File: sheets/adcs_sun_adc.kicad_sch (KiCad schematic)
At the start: 1 part, among them U10 MCP3208

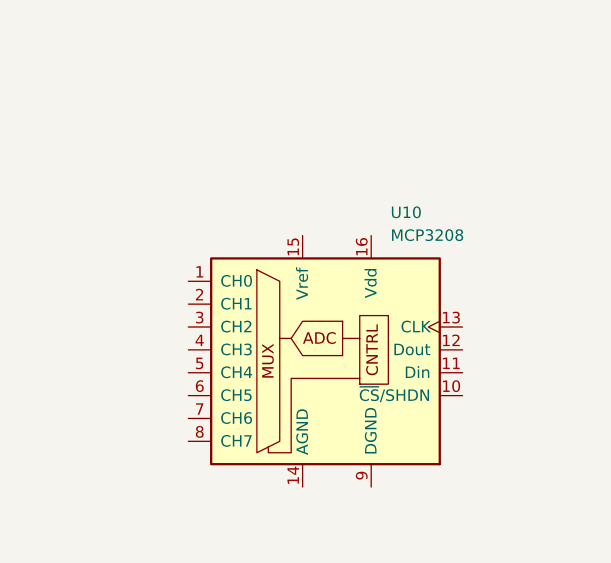
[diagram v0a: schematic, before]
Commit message: push
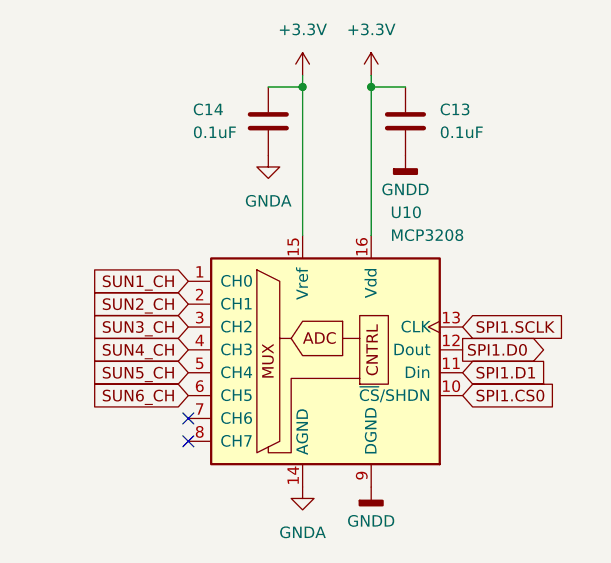
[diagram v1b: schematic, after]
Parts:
- added C13, C14: 0.1uF, symbol Device:C
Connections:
- net SUN1_CH: now reaches U10.1 (CH0)
- net SPI1.CS0: now reaches U10.10 (~{CS}/SHDN)
- net SPI1.D1: now reaches U10.11 (Din)
- net SPI1.D0: now reaches U10.12 (Dout)
- net SPI1.SCLK: now reaches U10.13 (CLK)
- net GNDA: now reaches U10.14 (AGND)
- net GNDA: now also C14.2
- net +3.3V: now reaches U10.15 (Vref)
- net +3.3V: now also U10.16 (Vdd), C13.1, C14.1
- net SUN2_CH: now reaches U10.2 (CH1)
- net SUN3_CH: now reaches U10.3 (CH2)
- net SUN4_CH: now reaches U10.4 (CH3)
- net SUN5_CH: now reaches U10.5 (CH4)
- net SUN6_CH: now reaches U10.6 (CH5)
- net GNDD: now reaches U10.9 (DGND)
- net GNDD: now also C13.2
- no-connect marks 0 -> 2

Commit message: allocating pins ?
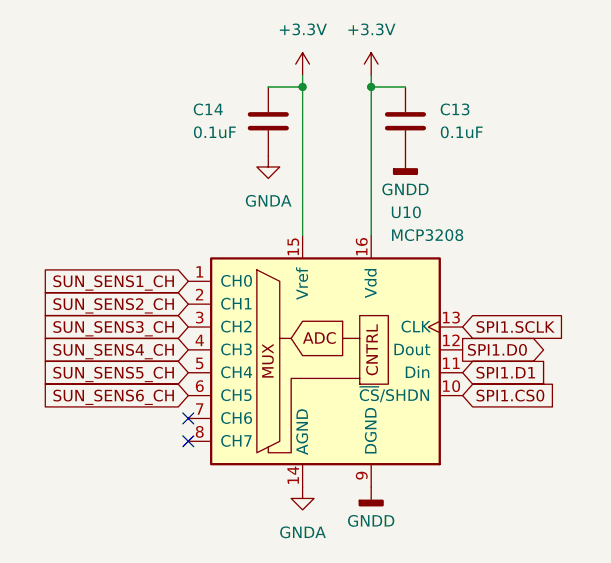
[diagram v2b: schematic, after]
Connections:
- net SUN1_CH renamed SUN_SENS1_CH
- net SUN2_CH renamed SUN_SENS2_CH
- net SUN3_CH renamed SUN_SENS3_CH
- net SUN4_CH renamed SUN_SENS4_CH
- net SUN5_CH renamed SUN_SENS5_CH
- net SUN6_CH renamed SUN_SENS6_CH
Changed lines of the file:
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@@
 		)
 	)
-	(global_label "SUN4_CH"
+	(global_label "SUN_SENS4_CH"
 		(shape input)
 		(at 133.35 91.44 180)
@@
 		)
 		(property "Intersheetrefs" "${INTERSHEET_REFS}"
-			(at 121.6216 91.44 0)
-			(hide yes)
-			(show_name no)
-			(do_not_autoplace no)
-			(effects
-				(font
-					(size 1.27 1.27)
-				)
-				(justify right)
-			)
-		)
-	)
-	(global_label "SUN6_CH"
+			(at 115.7555 91.44 0)
+			(hide yes)
+			(show_name no)
+			(do_not_autoplace no)
+			(effects
+				(font
+					(size 1.27 1.27)
+				)
+				(justify right)
+			)
+		)
+	)
+	(global_label "SUN_SENS6_CH"
 		(shape input)
 		(at 133.35 96.52 180)
@@
 		)
 		(property "Intersheetrefs" "${INTERSHEET_REFS}"
-			(at 121.6216 96.52 0)
-			(hide yes)
-			(show_name no)
-			(do_not_autoplace no)
-			(effects
-				(font
-					(size 1.27 1.27)
-				)
-				(justify right)
-			)
-		)
-	)
-	(global_label "SUN2_CH"
+			(at 115.7555 96.52 0)
+			(hide yes)
+			(show_name no)
+			(do_not_autoplace no)
+			(effects
+				(font
+					(size 1.27 1.27)
+				)
+				(justify right)
+			)
+		)
+	)
+	(global_label "SUN_SENS2_CH"
 		(shape input)
 		(at 133.35 86.36 180)
@@
 		)
 		(property "Intersheetrefs" "${INTERSHEET_REFS}"
-			(at 121.6216 86.36 0)
+			(at 115.7555 86.36 0)
 			(hide yes)
 			(show_name no)
@@
 		)
 	)
-	(global_label "SUN3_CH"
+	(global_label "SUN_SENS3_CH"
 		(shape input)
 		(at 133.35 88.9 180)
@@
 		)
 		(property "Intersheetrefs" "${INTERSHEET_REFS}"
-			(at 121.6216 88.9 0)
-			(hide yes)
-			(show_name no)
-			(do_not_autoplace no)
-			(effects
-				(font
-					(size 1.27 1.27)
-				)
-				(justify right)
-			)
-		)
-	)
-	(global_label "SUN5_CH"
+			(at 115.7555 88.9 0)
+			(hide yes)
+			(show_name no)
+			(do_not_autoplace no)
+			(effects
+				(font
+					(size 1.27 1.27)
+				)
+				(justify right)
+			)
+		)
+	)
+	(global_label "SUN_SENS5_CH"
 		(shape input)
 		(at 133.35 93.98 180)
@@
 		)
 		(property "Intersheetrefs" "${INTERSHEET_REFS}"
-			(at 121.6216 93.98 0)
+			(at 115.7555 93.98 0)
 			(hide yes)
 			(show_name no)
@@
 		)
 	)
-	(global_label "SUN1_CH"
+	(global_label "SUN_SENS1_CH"
 		(shape input)
 		(at 133.35 83.82 180)
@@
 		)
 		(property "Intersheetrefs" "${INTERSHEET_REFS}"
-			(at 121.6216 83.82 0)
-			(hide yes)
-			(show_name no)
+			(at 115.7555 83.82 0)
+			(hide yes)
+			(show_name no)
